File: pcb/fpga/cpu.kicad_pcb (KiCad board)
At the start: 2 copper layers, 76.2 x 50.8 mm, 58 parts, among them CON1 USB-MINI-B, P1 PWR, P2 BANK3, P3 BANK1, P4 BANK2, P5 BANK4, P6 CONN_6, U1 EPCS1, U2 LMS1585/7, U3 LM1084IS-3.3/NOPB, U4 EP1C3T100

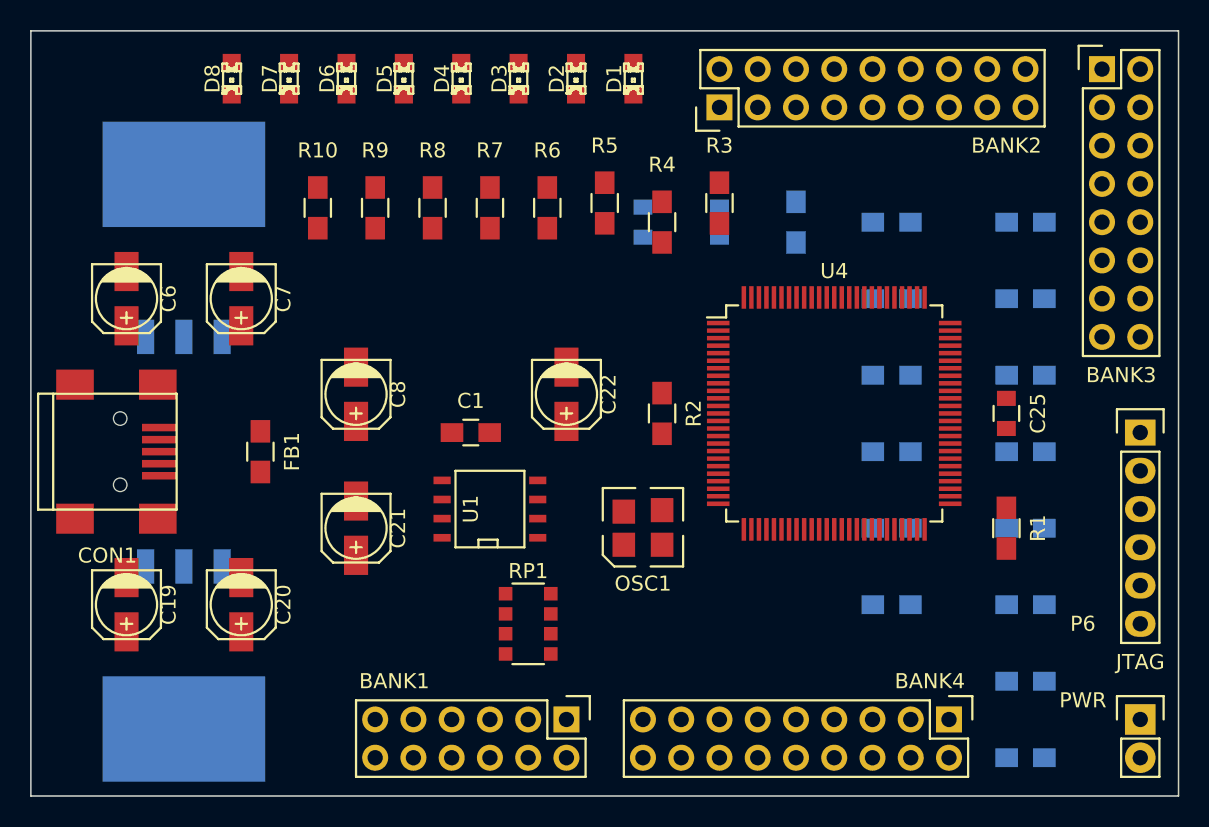
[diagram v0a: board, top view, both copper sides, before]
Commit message: Layout changes
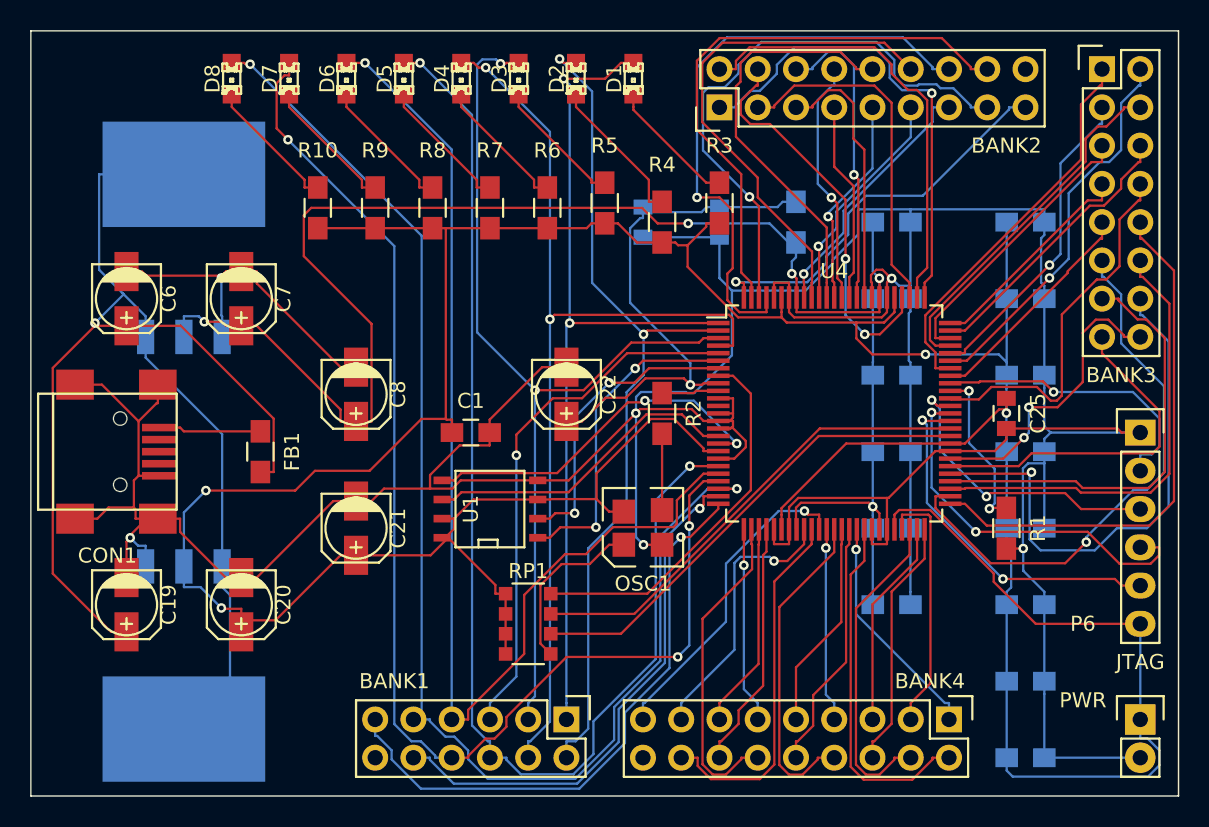
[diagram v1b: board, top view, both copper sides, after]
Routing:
- net GND: track 0.00 -> 289.4 mm, vias 0 -> 5
- net +3.3V: track 0.00 -> 255.2 mm, vias 0 -> 4
- net VCCINT: track 0.00 -> 114.1 mm, vias 0 -> 5
- net Net-(C19-Pad1): track 0.00 -> 93.2 mm, vias 0 -> 1
- net 2B13: track 0.00 -> 88.3 mm, vias 0 -> 2
- net 2B12: track 0.00 -> 84.1 mm, vias 0 -> 3
- net 2B10: track 0.00 -> 80.8 mm, vias 0 -> 2
- net 2B11: track 0.00 -> 75.2 mm, vias 0 -> 1
- net 0B13: track 0.00 -> 65.2 mm, vias 0 -> 2
- net 0B12: track 0.00 -> 61.9 mm, vias 0 -> 2
- net 0B10: track 0.00 -> 57.7 mm, vias 0 -> 2
- net 0B11: track 0.00 -> 57.4 mm, vias 0 -> 2
- net 2B23: track 0.00 -> 39.9 mm, vias 0 -> 1
- net 2B15: track 0.00 -> 39.5 mm, vias 0 -> 1
- net 2B24: track 0.00 -> 38.3 mm, vias 0 -> 1
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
